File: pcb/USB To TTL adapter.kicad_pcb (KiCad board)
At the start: 2 copper layers, 60 x 31 mm, 23 parts, among them J1 USB_B, J2 Conn_01x04, Q1 BC817, Q2 BC817, U1 CH340G, U2 PC817, U3 PC817, Y1 12 MHz

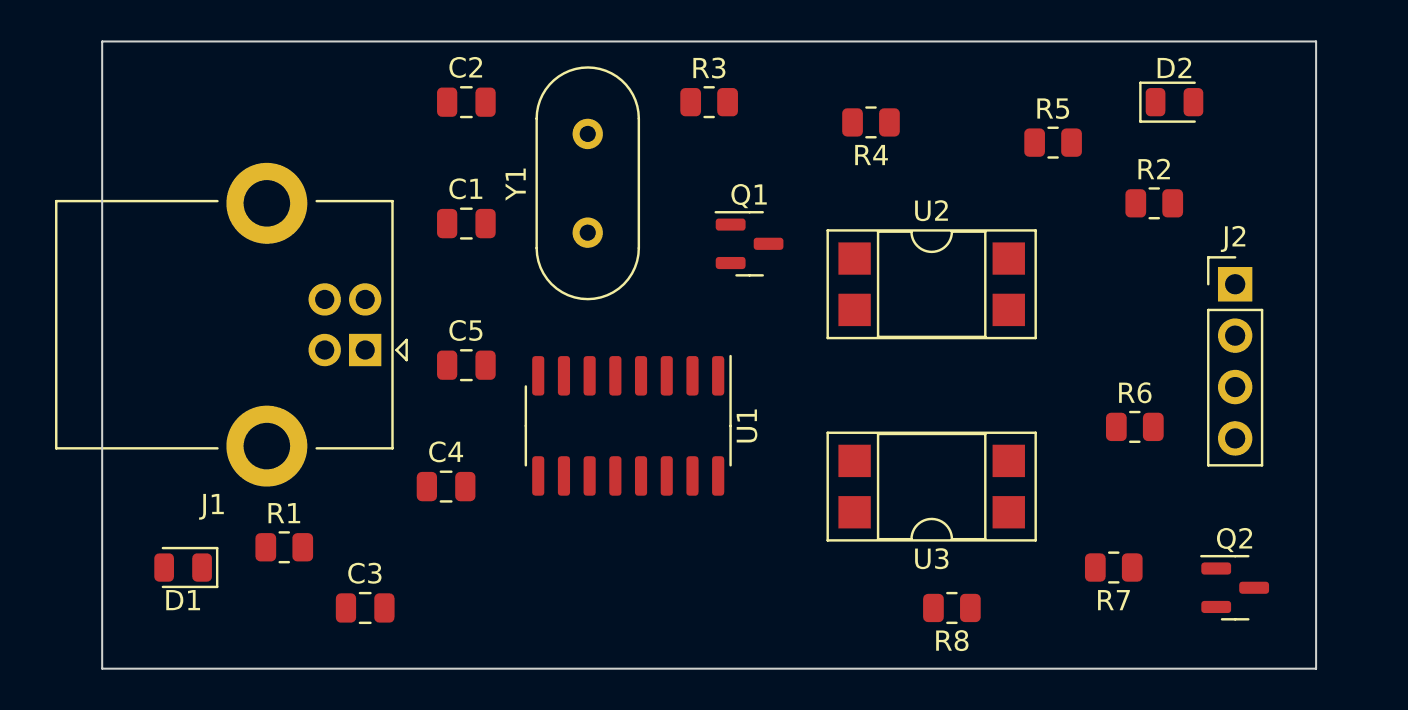
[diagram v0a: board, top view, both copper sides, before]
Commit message: Diseño de PCB
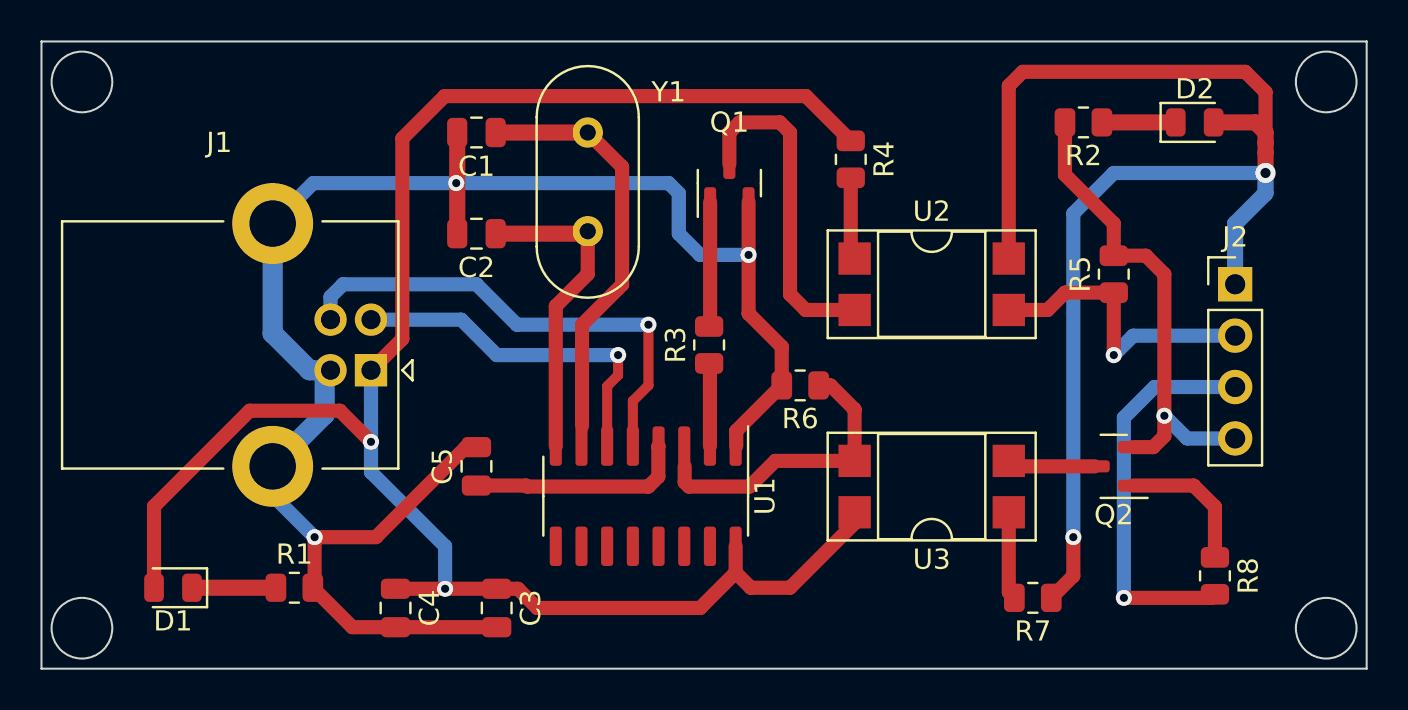
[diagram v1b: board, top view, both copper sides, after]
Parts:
- moved R6 16.7 mm to (152.5, 87.0), turned to 180 degrees
- moved R8 13.1 mm to (173.0, 96.4), turned to -90 degrees
- moved R3 12.0 mm to (148.0, 85.0), turned to 90 degrees
- moved Q2 8.49 mm to (168.0, 91.0), turned to 180 degrees
- moved R5 7.16 mm to (168.0, 81.5), turned to 90 degrees
- moved C2 6.52 mm to (136.5, 79.5), turned to 180 degrees
- moved C3 6.50 mm to (137.5, 98.0), turned to -90 degrees
- moved C4 6.50 mm to (132.5, 98.0), turned to -90 degrees
- moved R2 5.32 mm to (166.5, 74.0), turned to 180 degrees
- moved C5 5.02 mm to (136.5, 91.0), turned to 90 degrees
- moved Y1 4.95 mm to (142.0, 74.5), turned to -90 degrees
- moved C1 4.53 mm to (136.5, 74.5), turned to 180 degrees
- moved R7 4.27 mm to (164.0, 97.5)
- moved U1 3.58 mm to (144.9, 92.5)
- moved Q1 3.16 mm to (149.0, 77.0), turned to 90 degrees
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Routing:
- net VCC: track 0.00 -> 93.0 mm, vias 0 -> 2
- net GND: track 0.00 -> 87.3 mm, vias 0 -> 3
- net VDD: track 0.00 -> 64.6 mm, vias 0 -> 2
- net Net-(J1-Pad3): track 0.00 -> 24.2 mm, vias 0 -> 1
- net GND1: track 0.00 -> 24.2 mm, vias 0 -> 1
- net Net-(C1-Pad1): track 0.00 -> 20.6 mm
- net Net-(J2-Pad3): track 0.00 -> 19.6 mm, vias 0 -> 1
- net Net-(J1-Pad2): track 0.00 -> 17.7 mm, vias 0 -> 1
- net Net-(Q1-Pad3): track 0.00 -> 16.5 mm
- net Net-(C2-Pad1): track 0.00 -> 15.9 mm
- net Net-(J2-Pad2): track 0.00 -> 15.0 mm, vias 0 -> 1
- net Net-(R6-Pad1): track 0.00 -> 14.6 mm
- net /V3: track 0.00 -> 10.7 mm
- net Net-(Q2-Pad1): track 0.00 -> 7.00 mm
- net Net-(Q1-Pad1): track 0.00 -> 6.17 mm
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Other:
- board size 60 x 31 mm -> 65.5 x 31 mm
- board text added: "Emiliano Rodriguez - DCI - CESE"
- board text added: "USB To TTL Isolated"
